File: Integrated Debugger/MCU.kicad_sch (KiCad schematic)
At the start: 15 parts, among them SW1 BOOT, U2 STM32F103CBUx, Y1 8MHz

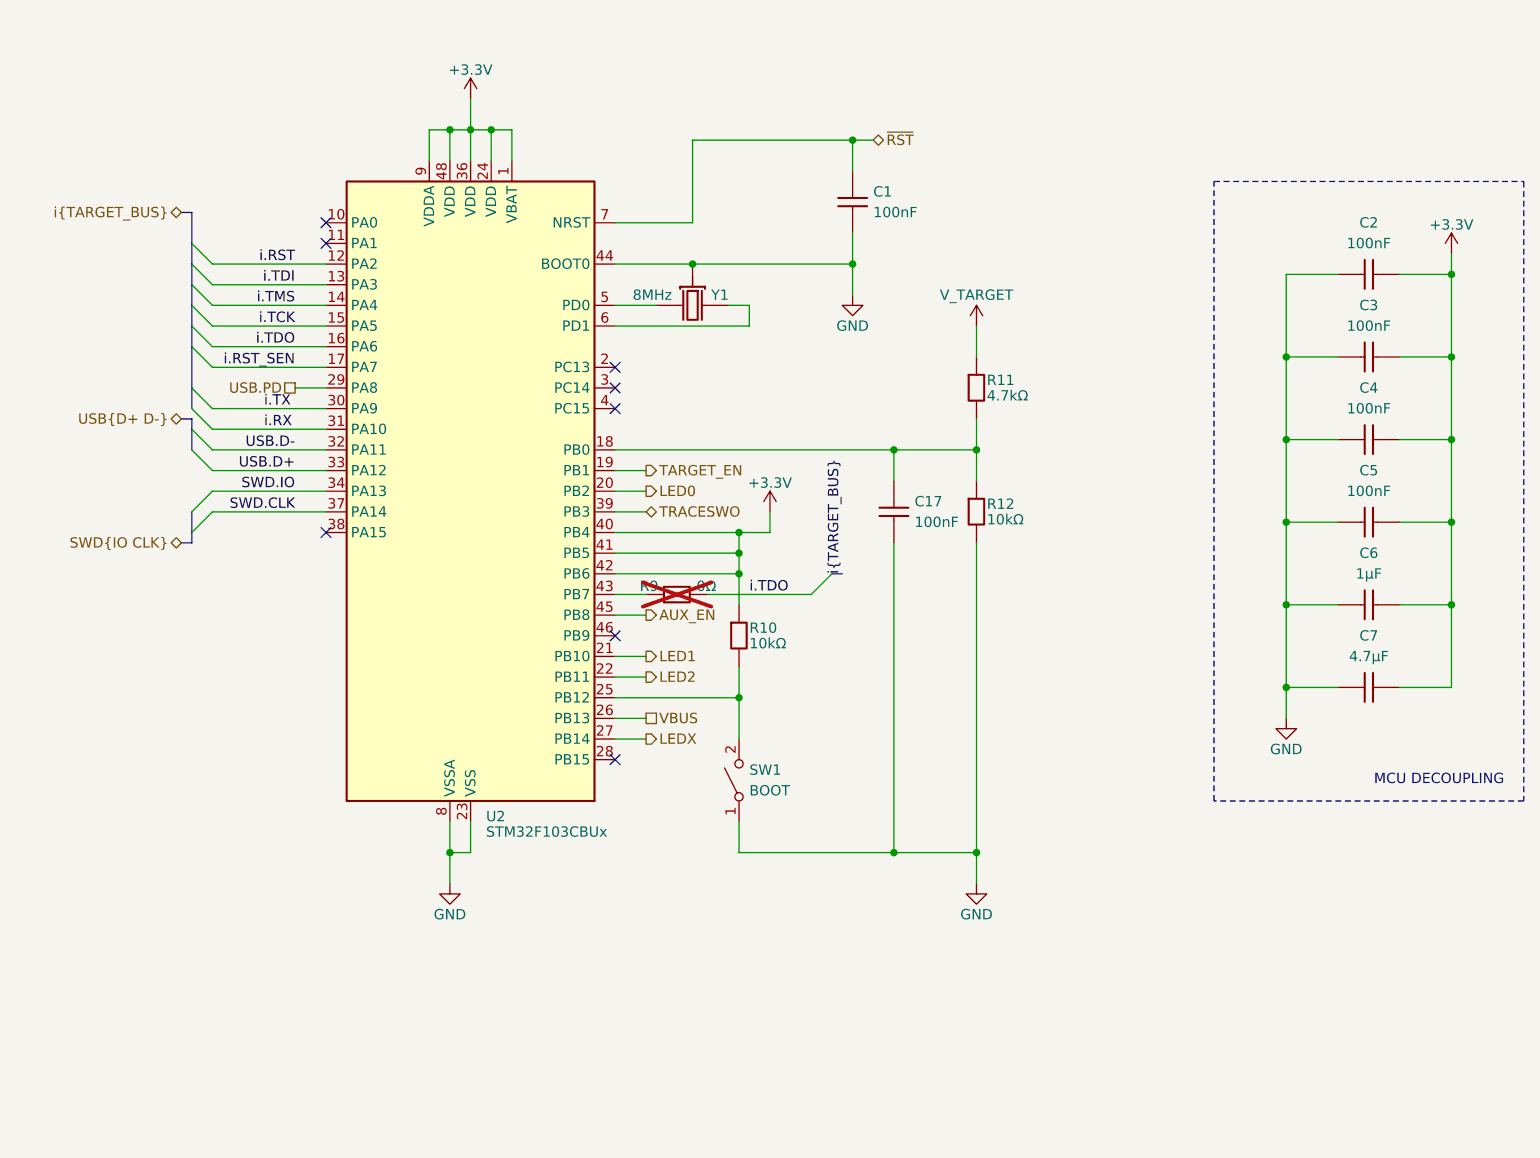
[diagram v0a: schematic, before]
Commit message: IDBG schematic
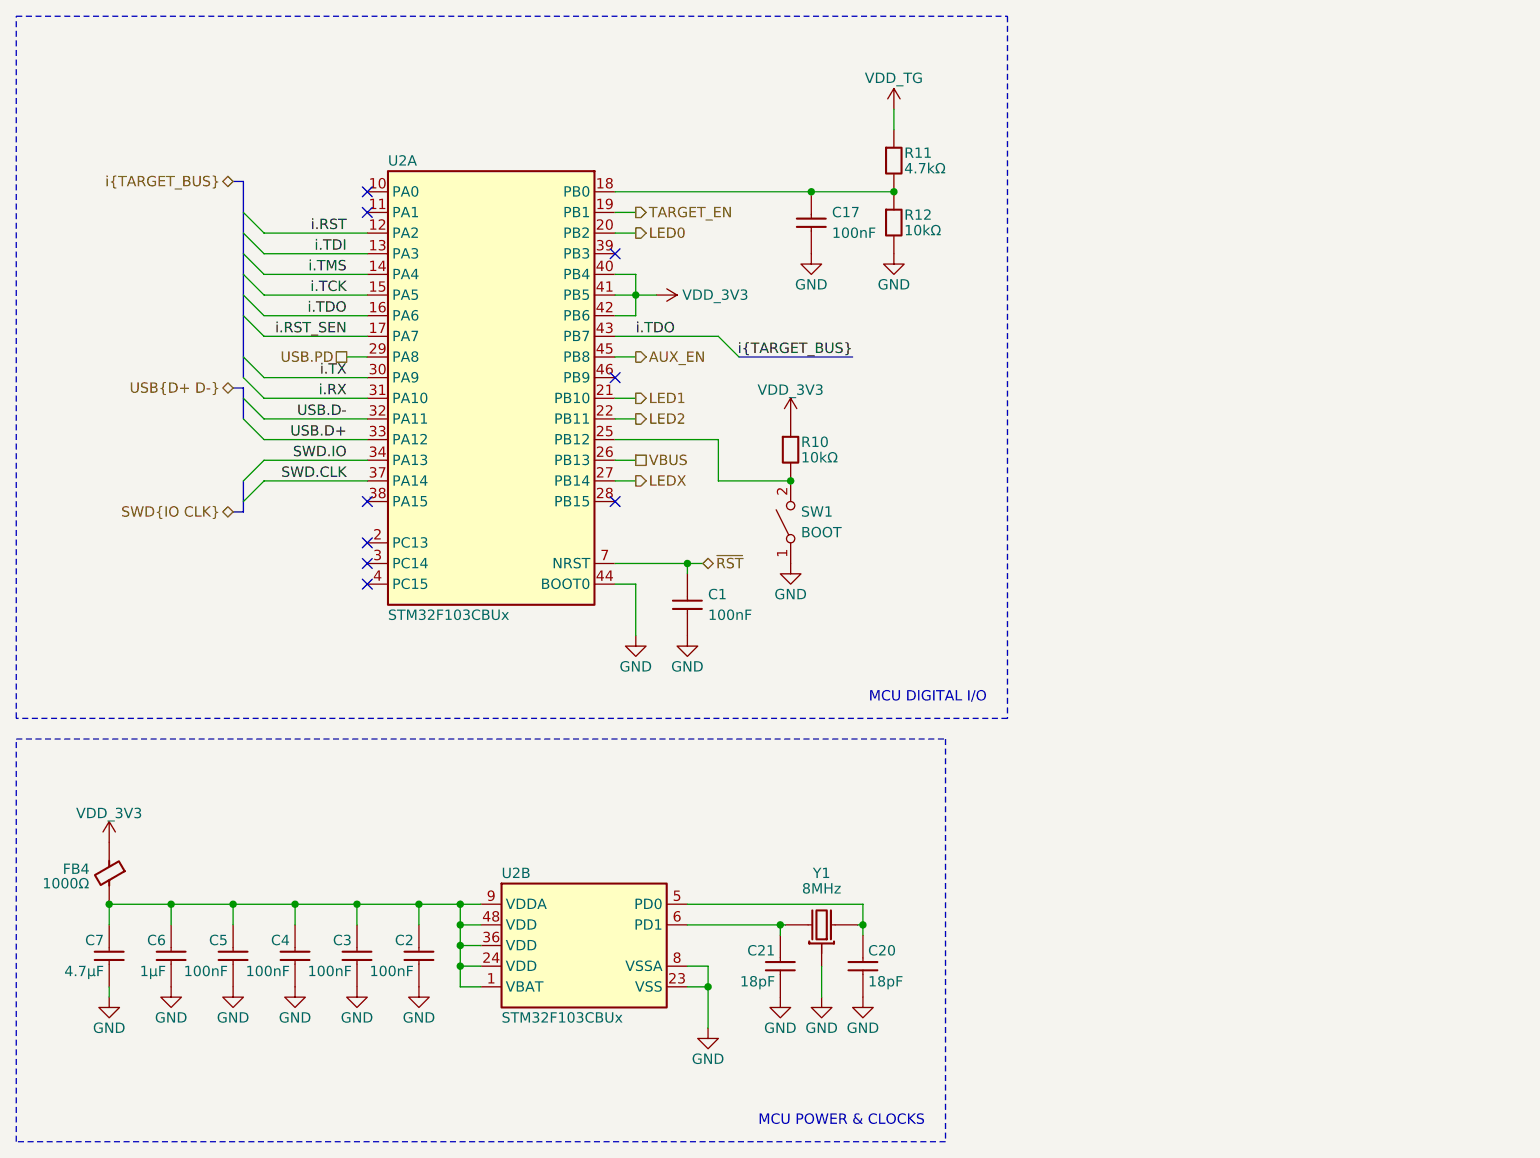
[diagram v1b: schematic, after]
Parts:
- removed R9: 0Ω, Picoballoon Passives:Resistor 0201, symbol Picoballoon Passives:Resistor
- added C20, C21: 18pF, Picoballoon Passives:Capacitor 0201, symbol Picoballoon Passives:Capacitor
- added FB4: 1000Ω, Picoballoon Passives:Inductor 0402, symbol Picoballoon Passives:Ferrite bead
- added unit 2 of U2
- C1, C17, C2, C3, C4, C5: JLCPCB Part # C76934 -> (none)
- C6: JLCPCB Part # C76930 -> (none)
- C7: JLCPCB Part # C335103 -> (none)
- R10, R12: JLCPCB Part # C717002 -> (none)
- R11: JLCPCB Part # C138135 -> (none)
- U2: JLCPCB Part # C55506 -> (none)
- Y1: footprint Picoballoon Passives:Crystal 3213-3P -> Picoballoon Passives:Crystal 3225; JLCPCB Part # C341525 -> (none); LCSC Part # C341525 -> C57131; MPN CSTNE8M00GH5C000R0 -> 1C208000BC0R
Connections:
- net GND: now also C20.1, C21.1, U2.23 (VSS), U2.35 (VSS), U2.47 (VSS), U2.49 (VSS), U2.8 (VSSA); no longer U2.23 (VSS), U2.35 (VSS), U2.47 (VSS), U2.49 (VSS), U2.8 (VSSA)
- net i.TDO: now also U2.43 (PB7)
- net at Y1.3: now also C21.2, U2.6 (PD1); no longer U2.5 (PD0)
- net at Y1.1: now also C20.2, U2.5 (PD0); no longer U2.6 (PD1)
- removed net +3.3V: C2.2, C3.2, C4.2, C5.2, C6.2, C7.2, R10.1, U2.1 (VBAT), U2.24 (VDD), U2.36 (VDD), U2.40 (PB4), U2.41 (PB5), U2.42 (PB6), U2.48 (VDD), U2.9 (VDDA)
- net TRACESWO: no longer names the net of U2.39 (PB3)
- net V_TARGET renamed VDD_TG
- new net: C2.2, C3.2, C4.2, C5.2, C6.2, C7.2, FB4.2, U2.1 (VBAT), U2.24 (VDD), U2.36 (VDD), U2.48 (VDD), U2.9 (VDDA)
- new net VDD_3V3: FB4.1, R10.1, U2.40 (PB4), U2.41 (PB5), U2.42 (PB6)
- no-connect marks 8 -> 9
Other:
- note added: "MCU DIGITAL I/O"
- note added: "MCU POWER & CLOCKS"
- note removed: "MCU DECOUPLING"
- moved on the sheet: C1, C17, C2, C3, C4, C5, C6, C7, R10, R11, R12, SW1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
